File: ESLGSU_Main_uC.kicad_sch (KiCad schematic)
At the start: 35 parts, among them U29 TCAN1051GVDRBRQ, U30 THVD1450DRBR, U31 TXU0304RUTR, U32 TS5A23159RSER, U33 TXU0202DTTR, U34 74LVC2G53GT, U35 TXU0202DTTR, U36 74LVC2G53GT, U37 74LVC2G53GT, U38 TXU0304RUTR, U39 PCA9306, U40 74LVC2G53GT, U41 74LVC2G66GT

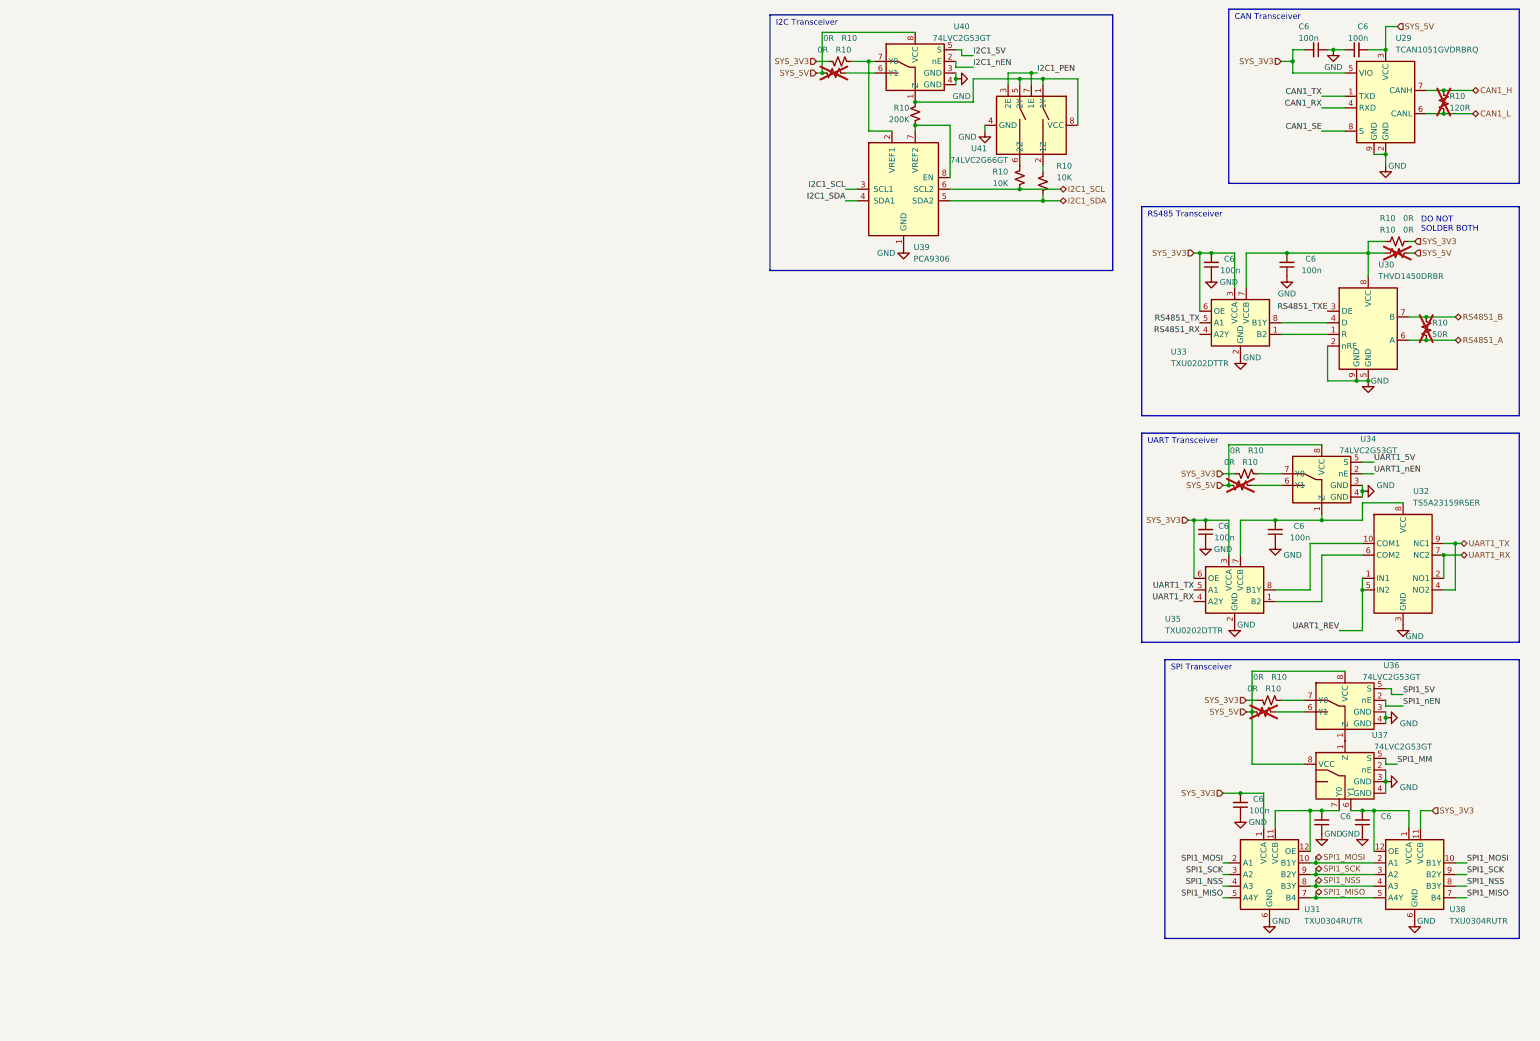
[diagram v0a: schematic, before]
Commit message: Finished interfaces work
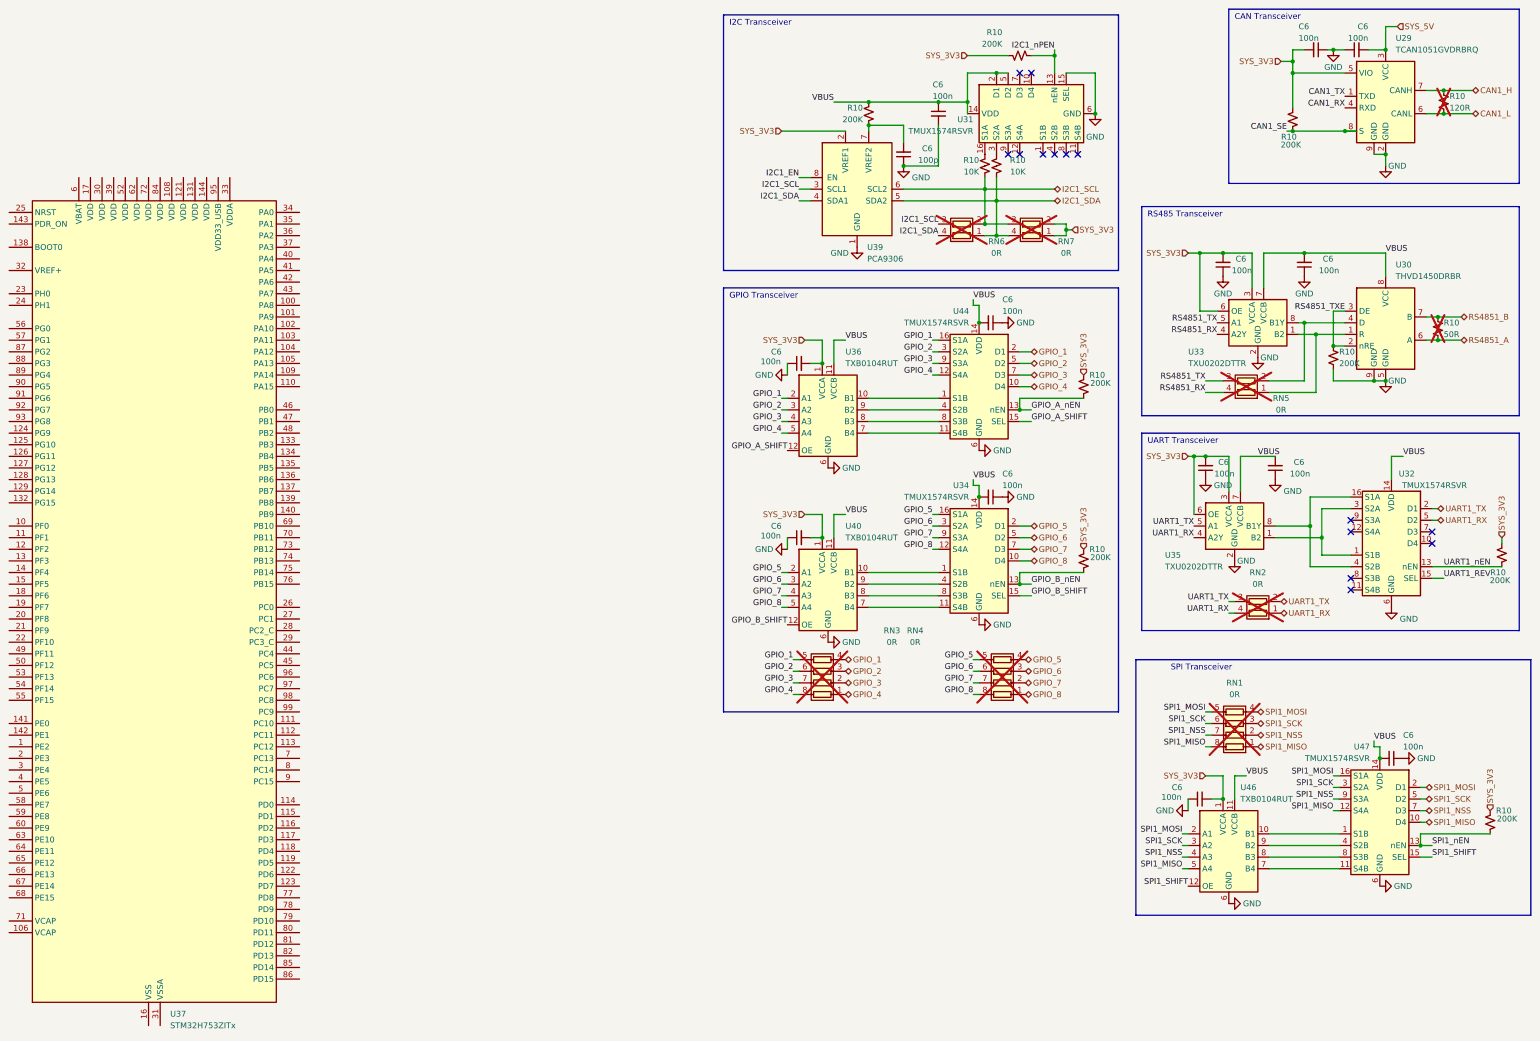
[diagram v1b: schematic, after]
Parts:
- removed C6 (x3): 100n, Capacitor_SMD:C_0603_1608Metric, symbol Device:C_Small
- removed R10 (x8): 0R, Resistor_SMD:R_0603_1608Metric, symbol Device:R_Small_US
- removed U31, U38: TXU0304RUTR, ESLGSU_Parts_Lib:T-UQFN-12, symbol ESLGSU_Parts_Lib:TXU0304-Q1
- removed U32: TS5A23159RSER, Package_DFN_QFN:Texas_UQFN-10_1.5x2mm_P0.5mm, symbol ESLGSU_Parts_Lib:TS5A23159RSER
- removed U34, U36, U37, U40: 74LVC2G53GT, ESLGSU_Parts_Lib:SOT833-1-XSON8, symbol ESLGSU_Parts_Lib:74LVC2G53GT
- removed U41: 74LVC2G66GT, ESLGSU_Parts_Lib:SOT833-1-XSON8, symbol ESLGSU_Parts_Lib:74LVC2G66GT
- added C6: 100p, Capacitor_SMD:C_0402_1005Metric, symbol Device:C_Small
- added C6 (x7): 100n, Capacitor_SMD:C_0402_1005Metric, symbol Device:C_Small
- added R10 (x7): 200K, Resistor_SMD:R_0402_1005Metric, symbol Device:R_Small_US
- added RN1, RN3, RN4: 0R, Resistor_SMD:R_Array_Concave_4x0402, symbol Device:R_Pack04
- added RN2, RN5, RN6, RN7: 0R, Resistor_SMD:R_Array_Convex_2x0402, symbol Device:R_Pack02
- added U31, U32, U34, U44, U47: TMUX1574RSVR, ESLGSU_Parts_Lib:T-UQFN-16, symbol ESLGSU_Parts_Lib:TMUX1574RSVR
- added U36, U40, U46: TXB0104RUT, ESLGSU_Parts_Lib:T-UQFN-12, symbol ESLGSU_Parts_Lib:TXB0104RUTR
- added U37: STM32H753ZITx, Package_QFP:LQFP-144_20x20mm_P0.5mm, symbol MCU_ST_STM32H7:STM32H753ZITx
- C6: footprint Capacitor_SMD:C_0603_1608Metric -> Capacitor_SMD:C_0402_1005Metric
- R10: footprint Resistor_SMD:R_0603_1608Metric -> Resistor_SMD:R_0402_1005Metric
- U39: footprint (none) -> ESLGSU_Parts_Lib:SOT833-1-XSON8
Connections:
- net CAN1_SE: now also R10.1
- net GND: now also C6.1, C6.1, C6.1, C6.1, C6.1, C6.1, C6.1, C6.2, R10.2, U31.15 (SEL), U31.6 (GND), U32.6 (GND), U34.6 (GND), U36.6 (GND), U40.6 (GND), U44.6 (GND), U46.6 (GND), U47.6 (GND); no longer U30.2 (nRE)
- net I2C1_SCL: now also RN6.2 (R2.1), RN6.3 (R2.2), RN7.3 (R2.2)
- net I2C1_SDA: now also RN6.1 (R1.1), RN6.4 (R1.2), RN7.4 (R1.2)
- net RS4851_RX: now also RN5.4 (R1.2)
- net RS4851_TX: now also RN5.3 (R2.2)
- net RS4851_TXE: now also U30.2 (nRE), R10.1
- net SPI1_MISO: now also RN1.1 (R1.1), RN1.8 (R1.2), U46.5 (A4), U47.10 (D4), U47.12 (S4A)
- net SPI1_MOSI: now also RN1.4 (R4.1), RN1.5 (R4.2), U46.2 (A1), U47.16 (S1A), U47.2 (D1)
- net SPI1_NSS: now also RN1.2 (R2.1), RN1.7 (R2.2), U46.4 (A3), U47.7 (D3), U47.9 (S3A)
- net SPI1_SCK: now also RN1.3 (R3.1), RN1.6 (R3.2), U46.3 (A2), U47.3 (S2A), U47.5 (D2)
- net SPI1_nEN: now also R10.1, U47.13 (nEN)
- net SYS_3V3: now also U39.2 (VREF1), C6.2, C6.2, C6.2, R10.1, R10.2, R10.2, R10.2, R10.2, R10.2, RN7.1 (R1.1), RN7.2 (R2.1), U36.1 (VCCA), U40.1 (VCCA), U46.1 (VCCA)
- net UART1_REV: now also U32.15 (SEL)
- net UART1_RX: now also RN2.1 (R1.1), RN2.4 (R1.2), U32.5 (D2)
- net UART1_TX: now also RN2.2 (R2.1), RN2.3 (R2.2), U32.2 (D1)
- net UART1_nEN: now also R10.1, U32.13 (nEN)
- net VBUS: now reaches R10.1
- net VBUS: now also C6.2, C6.2, U30.8 (VCC), U33.7 (VCCB), U35.7 (VCCB), C6.1, C6.2, C6.2, C6.2, U31.14 (VDD), U31.2 (D1), U31.5 (D2), U32.14 (VDD), U34.14 (VDD), U36.11 (VCCB), U40.11 (VCCB), U44.14 (VDD), U46.11 (VCCB), U47.14 (VDD)
- net at R10.2, U39.7 (VREF2): now also C6.2; no longer U39.8 (EN)
- net at U30.1 (R), U33.1 (B2): now also RN5.1 (R1.1)
- net at U30.4 (D), U33.8 (B1Y): now also RN5.2 (R2.1)
- net at R10.1: now also U31.3 (S2A)
- net at R10.1: now also U31.16 (S1A)
- net at U35.1 (B2): now also U32.1 (S1B), U32.3 (S2A)
- net at U35.8 (B1Y): now also U32.16 (S1A), U32.4 (S2B)
- new net: U46.10 (B1), U47.1 (S1B)
- new net: U46.7 (B4), U47.11 (S4B)
- new net: U46.9 (B2), U47.4 (S2B)
- new net: U46.8 (B3), U47.8 (S3B)
- new net: U36.10 (B1), U44.1 (S1B)
- new net: U36.7 (B4), U44.11 (S4B)
- new net: U36.9 (B2), U44.4 (S2B)
- new net: U36.8 (B3), U44.8 (S3B)
- new net: U34.1 (S1B), U40.10 (B1)
- new net: U34.11 (S4B), U40.7 (B4)
- new net: U34.8 (S3B), U40.8 (B3)
- new net: U34.4 (S2B), U40.9 (B2)
- new net: U37.107 (VSS), U37.120 (VSS), U37.130 (VSS), U37.16 (VSS), U37.38 (VSS), U37.51 (VSS), U37.61 (VSS), U37.83 (VSS), U37.94 (VSS)
- new net GPIO_1: RN3.4 (R4.1), RN3.5 (R4.2), U36.2 (A1), U44.16 (S1A), U44.2 (D1)
- new net GPIO_2: RN3.3 (R3.1), RN3.6 (R3.2), U36.3 (A2), U44.3 (S2A), U44.5 (D2)
- new net GPIO_3: RN3.2 (R2.1), RN3.7 (R2.2), U36.4 (A3), U44.7 (D3), U44.9 (S3A)
- new net GPIO_4: RN3.1 (R1.1), RN3.8 (R1.2), U36.5 (A4), U44.10 (D4), U44.12 (S4A)
- new net GPIO_5: RN4.4 (R4.1), RN4.5 (R4.2), U34.16 (S1A), U34.2 (D1), U40.2 (A1)
- new net GPIO_6: RN4.3 (R3.1), RN4.6 (R3.2), U34.3 (S2A), U34.5 (D2), U40.3 (A2)
- new net GPIO_7: RN4.2 (R2.1), RN4.7 (R2.2), U34.7 (D3), U34.9 (S3A), U40.4 (A3)
- new net GPIO_8: RN4.1 (R1.1), RN4.8 (R1.2), U34.10 (D4), U34.12 (S4A), U40.5 (A4)
- new net GPIO_A_SHIFT: U36.12 (OE), U44.15 (SEL)
- new net GPIO_A_nEN: R10.1, U44.13 (nEN)
- new net GPIO_B_SHIFT: U34.15 (SEL), U40.12 (OE)
- new net GPIO_B_nEN: R10.1, U34.13 (nEN)
- new net I2C1_EN: U39.8 (EN)
- new net I2C1_nPEN: R10.2, U31.13 (nEN)
- new net SPI1_SHIFT: U46.12 (OE), U47.15 (SEL)
- no-connect marks 0 -> 14
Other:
- note added: "GPIO Transceiver"
- note removed: "DO NOT SOLDER BOTH"
- moved on the sheet: C6, R10, U30, U33, U35, U39
